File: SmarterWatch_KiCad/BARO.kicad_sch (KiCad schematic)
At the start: 1 part

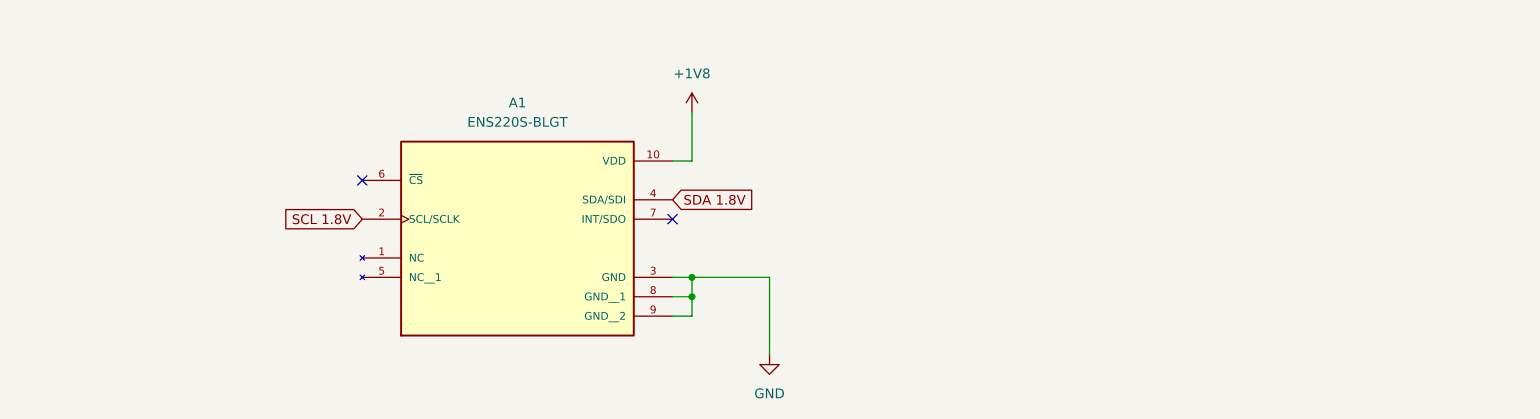
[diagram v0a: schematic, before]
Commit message: update
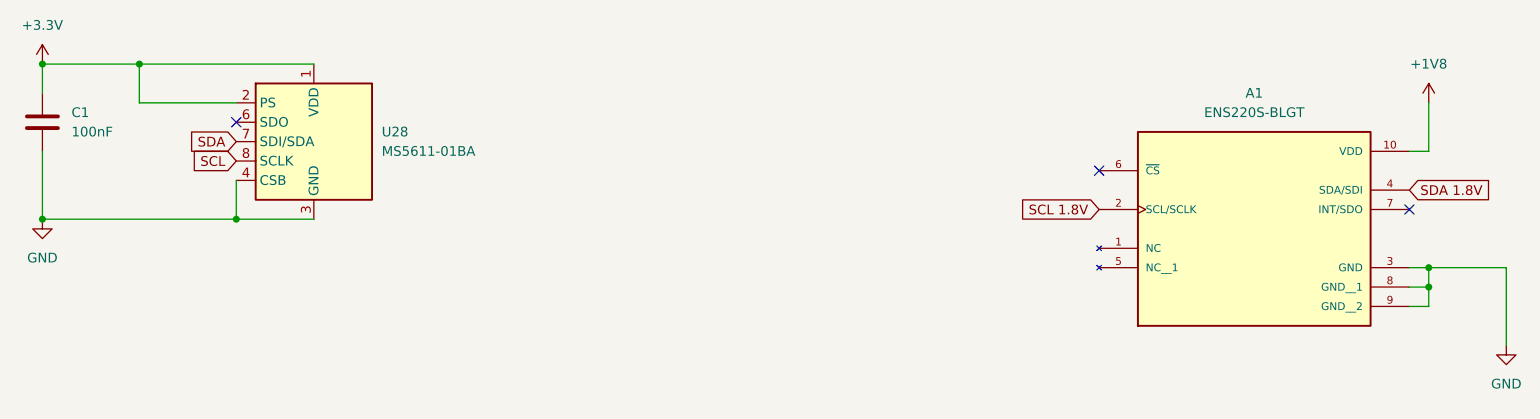
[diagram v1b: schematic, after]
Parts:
- added C1: 100nF, symbol Device:C
- added U28: MS5611-01BA, Package_LGA:LGA-8_3x5mm_P1.25mm, symbol Sensor_Pressure:MS5611-01BA
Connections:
- net GND: now also C1.2, U28.3 (GND), U28.4 (CSB), U28.5 (CSB)
- new net +3.3V: C1.1, U28.1 (VDD), U28.2 (PS)
- new net SCL: U28.8 (SCLK)
- new net SDA: U28.7 (SDI/SDA)
- no-connect marks 2 -> 3
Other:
- moved on the sheet: A1
